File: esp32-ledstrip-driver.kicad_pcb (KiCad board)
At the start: 2 copper layers, 43 parts, among them P1 PWR, P2 LED_1, P3 LED_2, P4 LED_3, P5 LED_4, P6 RS485, Q1 FDD8880?, Q2 FDD8880?, Q3 FDD8880?, Q4 FDD8880?, Q5 FDD8880?, Q6 FDD8880?, Q7 FDD8880?, Q8 FDD8880?, U1 ESP32-WROOM-32, U2 R-78E-1.0, U3 MAX481E

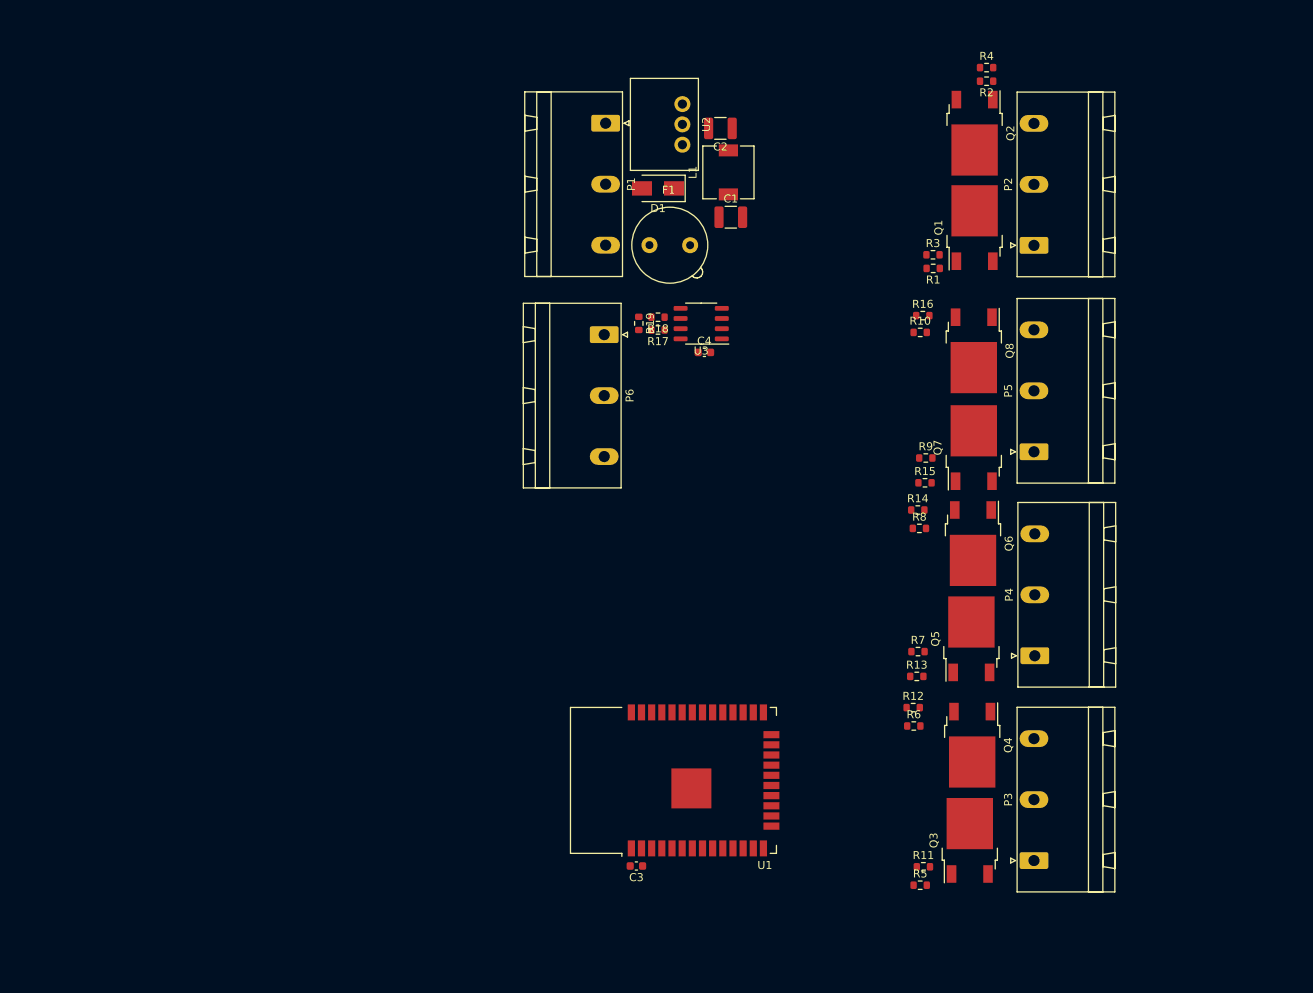
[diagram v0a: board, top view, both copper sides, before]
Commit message: first gerbers generated
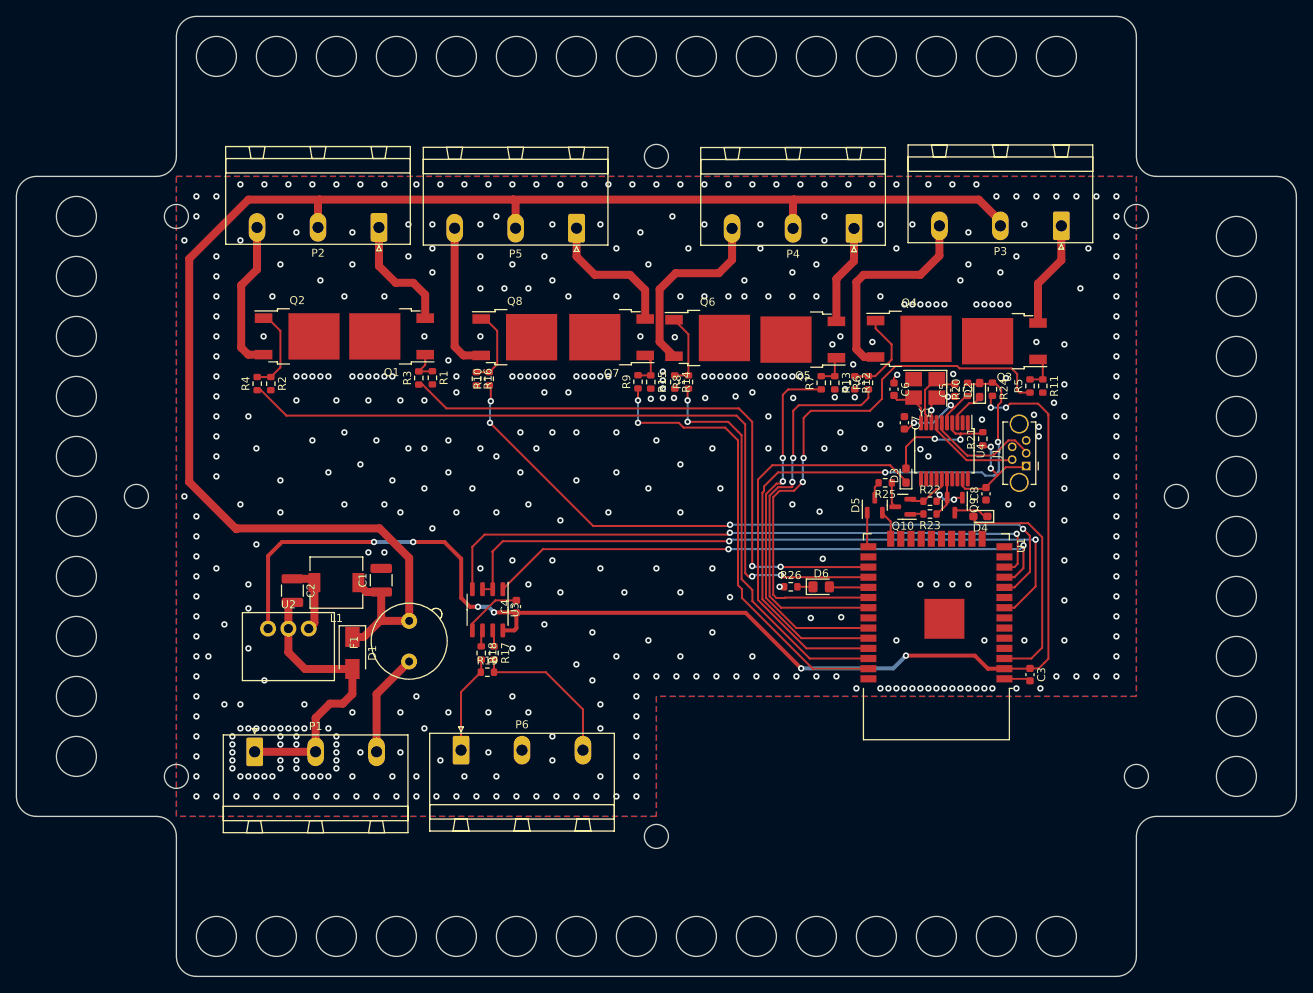
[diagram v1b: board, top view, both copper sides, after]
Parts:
- added C5: 20p, Capacitor_SMD:C_0603_1608Metric, F.Cu at (157.3, 81.7)
- added C6: 20p, Capacitor_SMD:C_0603_1608Metric, F.Cu at (149.7, 81.6)
- added C7: 100n, Capacitor_SMD:C_0603_1608Metric, F.Cu at (151.0, 85.8)
- added C8: 22u, Capacitor_SMD:C_0603_1608Metric, F.Cu at (161.2, 94.7)
- added D2: D_Schottky_Small, Diode_SMD:D_0603_1608Metric_Pad1.05x0.95mm_HandSolder, F.Cu at (160.4, 81.7)
- added D3: D_Schottky_Small, Diode_SMD:D_0603_1608Metric_Pad1.05x0.95mm_HandSolder, F.Cu at (151.2, 92.4)
- added D4: D_Schottky_Small, Diode_SMD:D_0603_1608Metric_Pad1.05x0.95mm_HandSolder, F.Cu at (160.5, 97.5)
- added D5: BAT54C, Package_TO_SOT_SMD:SOT-23, F.Cu at (147.3, 96.1)
- added D6: Led_Small, LED_SMD:LED_0805_2012Metric_Pad1.15x1.40mm_HandSolder, F.Cu at (140.6, 106.3)
- added J1: USB_B_Micro, Connector_USB:USB_Mini-B_Tensility_54-00023_Vertical_CircularHoles, F.Cu at (166.2, 91.2)
- added Q10: BC817, Package_TO_SOT_SMD:SOT-23, F.Cu at (150.8, 96.3)
- added Q9: BC817, Package_TO_SOT_SMD:SOT-23, F.Cu at (157.3, 96.1)
- added R20: 10k, Resistor_SMD:R_0603_1608Metric, F.Cu at (158.9, 81.6)
- added R21: 10k, Resistor_SMD:R_0603_1608Metric, F.Cu at (160.8, 87.8)
- added R22: 1k, Resistor_SMD:R_0603_1608Metric, F.Cu at (154.2, 95.6)
- added R23: 1k, Resistor_SMD:R_0603_1608Metric, F.Cu at (154.2, 97.2)
- added R24: DNP, Resistor_SMD:R_0603_1608Metric, F.Cu at (162.0, 81.6)
- added R25: 220R, Resistor_SMD:R_0603_1608Metric, F.Cu at (148.6, 93.3)
- added R26: 220R, Resistor_SMD:R_0603_1608Metric, F.Cu at (136.8, 106.3)
- added U4: CH340T, Package_SO:SSOP-20_5.3x7.2mm_P0.65mm, F.Cu at (156.0, 89.3)
- added Y1: Crystal_GND24_Small, Crystal:Crystal_SMD_3225-4Pin_3.2x2.5mm_HandSoldering, F.Cu at (153.6, 81.5)
- moved R4 99.4 mm to (70.1, 80.9), turned to 90 degrees
- moved R2 97.1 mm to (71.8, 80.9), turned to -90 degrees
- moved P1 90.0 mm to (69.8, 126.9), turned to 0 degrees
- moved Q2 88.4 mm to (75.1, 75.0), turned to 0 degrees
- moved P2 81.9 mm to (85.3, 61.4), turned to 180 degrees
- moved U2 80.0 mm to (74.0, 111.5), turned to 180 degrees
- moved P3 79.4 mm to (170.6, 61.2), turned to 180 degrees
- moved C2 78.7 mm to (74.5, 106.8), turned to -90 degrees
- moved Q1 74.1 mm to (86.9, 75.0), turned to 180 degrees
- moved L1 70.9 mm to (80.0, 105.8), turned to 180 degrees
- moved D1 69.5 mm to (82.0, 114.6), turned to -90 degrees
- moved R3 66.1 mm to (90.3, 80.2), turned to 90 degrees
- moved R1 64.1 mm to (92.0, 80.2), turned to -90 degrees
- moved R5 63.9 mm to (166.7, 81.2), turned to 90 degrees
- moved P5 63.6 mm to (110.0, 61.5), turned to 180 degrees
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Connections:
- R17 pad 2: Net-(P6-Pad1) -> Net-(P6-Pad3)
- R18 pad 2: Net-(P6-Pad3) -> Net-(P6-Pad1)
- R19 pad 1: Net-(P6-Pad3) -> Net-(P6-Pad1)
- R19 pad 2: Net-(P6-Pad1) -> Net-(P6-Pad3)
- U1 pad 11: unconnected-(U1-Pad11) -> RO
- U1 pad 12: unconnected-(U1-Pad12) -> DI
- U1 pad 24: unconnected-(U1-Pad24) -> GPIO_2
- U1 pad 25: unconnected-(U1-Pad25) -> GPIO_0
- U1 pad 29: unconnected-(U1-Pad29) -> Net-(D6-Pad2)
- U1 pad 3: unconnected-(U1-Pad3) -> ESP_EN
- U1 pad 34: unconnected-(U1-Pad34) -> RXD_0
- U1 pad 35: unconnected-(U1-Pad35) -> TXD_0
- U1 pad 8: unconnected-(U1-Pad8) -> ~{RX}TX
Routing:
- net +24V: track 0.00 -> 199.3 mm
- net +3V3: track 0.00 -> 162.2 mm, vias 0 -> 8
- net LED_1_W: track 0.00 -> 97.1 mm, vias 0 -> 2
- net LED_4_W: track 0.00 -> 86.8 mm, vias 0 -> 4
- net ~{RX}TX: track 0.00 -> 85.4 mm, vias 0 -> 2
- net DI: track 0.00 -> 79.8 mm, vias 0 -> 2
- net LED_1_C: track 0.00 -> 76.2 mm, vias 0 -> 2
- net RXD_0: track 0.00 -> 74.9 mm, vias 0 -> 2
- net RO: track 0.00 -> 73.0 mm, vias 0 -> 2
- net LED_2_C: track 0.00 -> 71.8 mm, vias 0 -> 2
- net LED_4_C: track 0.00 -> 57.1 mm, vias 0 -> 2
- net GND: track 0.00 -> 54.4 mm, vias 0 -> 471
- net TXD_0: track 0.00 -> 51.7 mm
- net LED_3_W: track 0.00 -> 50.4 mm, vias 0 -> 2
- net LED_2_W: track 0.00 -> 49.5 mm, vias 0 -> 2
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- added copper zone on B.Cu, net GND
- added copper zone on F.Cu, net GND
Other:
- board outline added: 160 x 120 mm
